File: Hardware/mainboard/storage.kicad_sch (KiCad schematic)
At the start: 11 parts, among them J502 SD_Card, U301 MIMXRT1176DVMAA, U501 W25Q128JWP

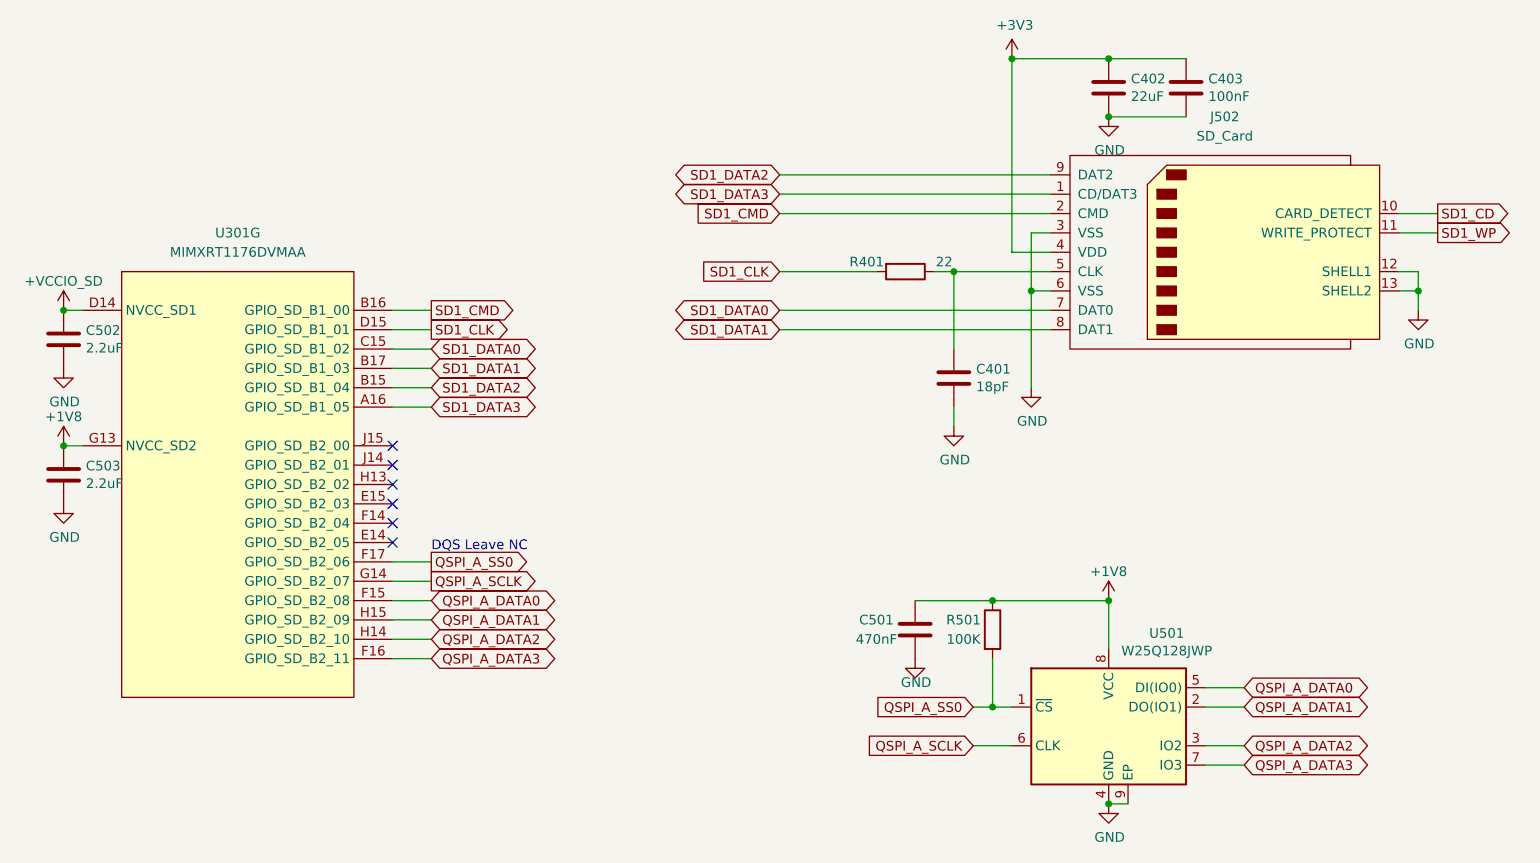
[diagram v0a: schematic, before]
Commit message: New mainboard rev wip
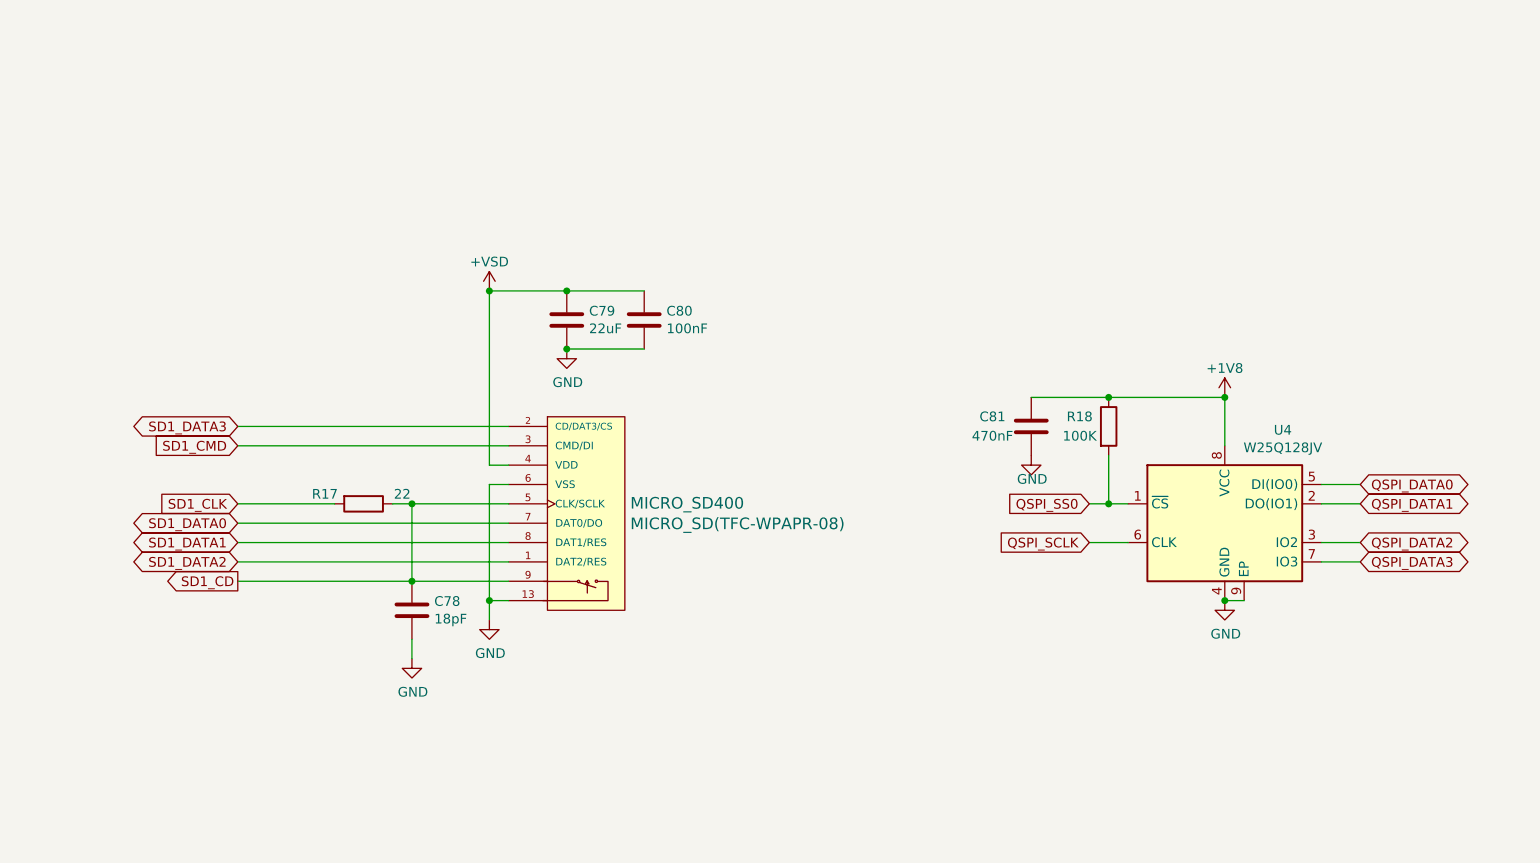
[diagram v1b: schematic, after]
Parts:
- removed C502, C503: 2.2uF, Capacitor_SMD:C_0402_1005Metric, symbol Device:C
- removed J502: SD_Card, Connector_Card:SD_Kyocera_145638009511859+, symbol Connector:SD_Card
- removed U301: MIMXRT1176DVMAA, footprints:BGA-289_17x17_14.0x14.0mm, symbol symbols:MIMXRT1176DVMAA
- added MICRO_SD400: MICRO_SD(TFC-WPAPR-08), footprints:TFC-WPAPR-08, symbol Sitina:MICRO_SD(TFC-WPAPR-08)
- U4: renamed from U501; value W25Q128JWP -> W25Q128JV
- renumbered C401 to C78, C402 to C79, C403 to C80, C501 to C81, R401 to R17, R501 to R18
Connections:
- net GND: now also MICRO_SD400.10, MICRO_SD400.11, MICRO_SD400.12, MICRO_SD400.13, MICRO_SD400.6 (VSS)
- net SD1_CD: now also C78.1, R17.1, MICRO_SD400.5 (CLK/SCLK), MICRO_SD400.9
- net SD1_CMD: now also MICRO_SD400.3 (CMD/DI)
- net SD1_DATA0: now also MICRO_SD400.7 (DAT0/DO)
- net SD1_DATA1: now also MICRO_SD400.8 (DAT1/RES)
- net SD1_DATA2: now also MICRO_SD400.1 (DAT2/RES)
- net SD1_DATA3: now also MICRO_SD400.2 (CD/DAT3/CS)
- net +3V3 renamed +VSD
- net +VSD: now also MICRO_SD400.4 (VDD)
- net QSPI_A_DATA0 renamed QSPI_DATA0
- net QSPI_A_DATA1 renamed QSPI_DATA1
- net QSPI_A_DATA2 renamed QSPI_DATA2
- net QSPI_A_DATA3 renamed QSPI_DATA3
- net QSPI_A_SCLK renamed QSPI_SCLK
- net QSPI_A_SS0 renamed QSPI_SS0
- no-connect marks 6 -> 0
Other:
- note removed: "DQS Leave NC"
- moved on the sheet: C78, C79, C80, C81, R17, R18, U4
